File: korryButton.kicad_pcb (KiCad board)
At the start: 2 copper layers, 30 x 30 mm, 15 parts, among them CN1 B2B-XH-A (LF)(SN), CN2 B2B-XH-A (LF)(SN), SW1 5.8 ZSGT, U1 SN74AHCT125DR, U2 B3B-XH-A(LF)(SN), U3 WS2811C, U4 WS2811C

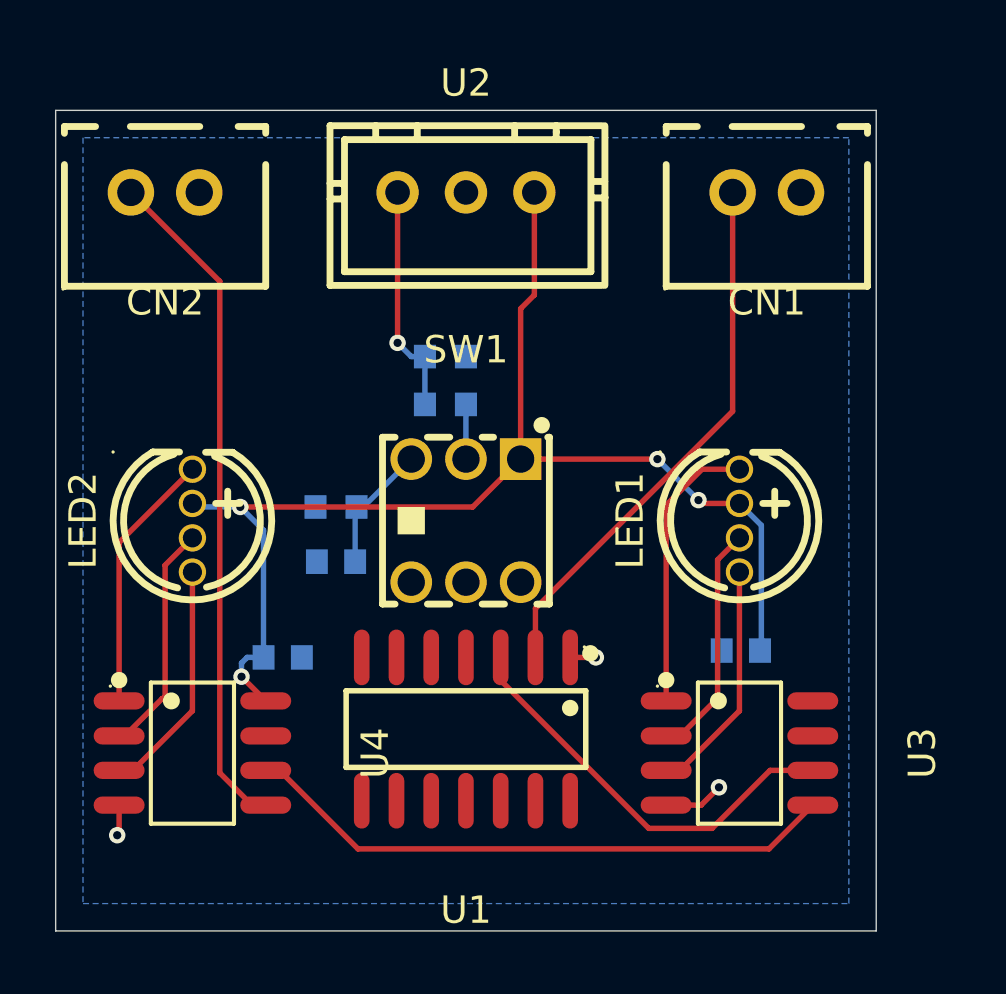
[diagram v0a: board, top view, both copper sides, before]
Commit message: update pcb
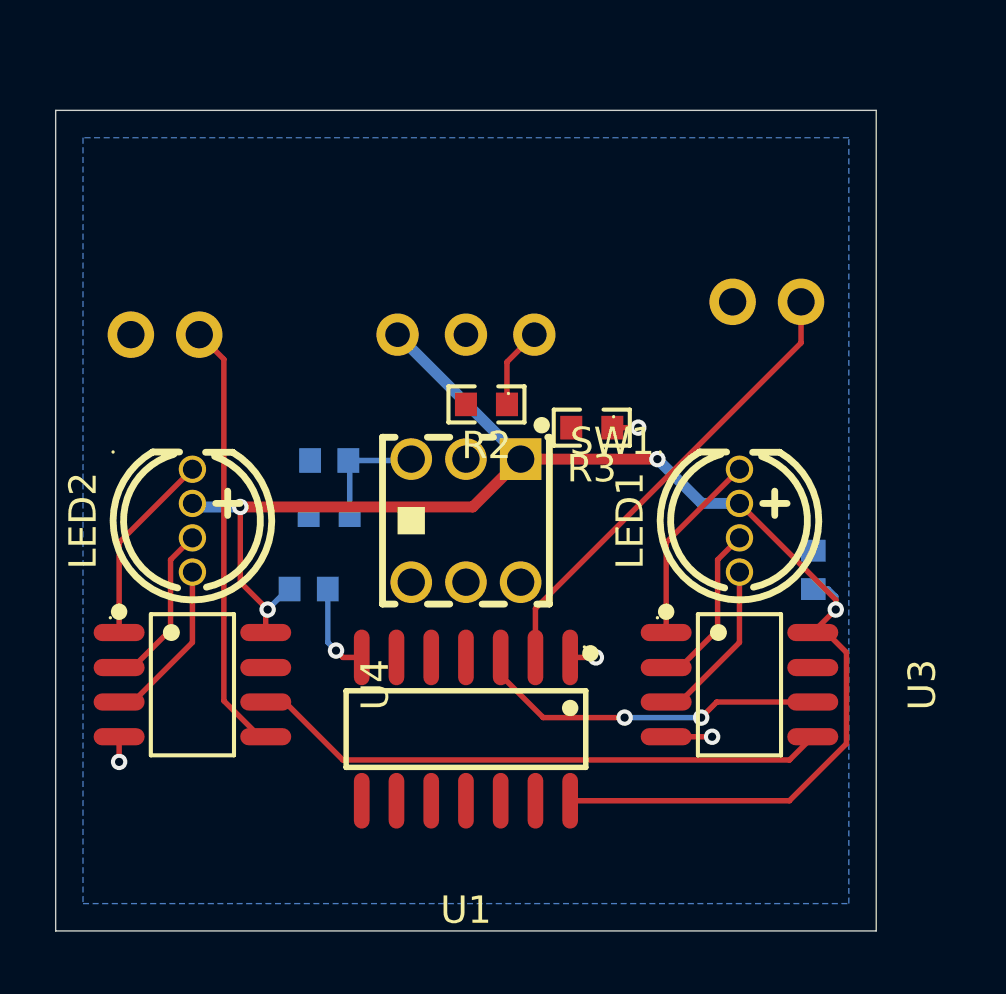
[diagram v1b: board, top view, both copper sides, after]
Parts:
- CN1, CN2, U2: moved to B.Cu
- R2, R3: moved to F.Cu
- moved R3 5.95 mm to (104.6, 121.6)
- moved CN2 5.20 mm to (89.0, 118.2), turned to 0 degrees
- moved U2 5.20 mm to (100.0, 118.2), turned to 180 degrees
- moved CN1 4.00 mm to (111.0, 117.0), turned to 0 degrees
- moved C3 3.97 mm to (112.7, 126.8), turned to -90 degrees
- moved C1 3.71 mm to (95.0, 122.8)
- moved C2 2.67 mm to (94.2, 127.5)
- moved U3 2.50 mm to (110.0, 131.0)
- moved U4 2.50 mm to (90.0, 131.0)
- moved R2 1.50 mm to (100.8, 120.8), turned to 180 degrees
- moved R1 0.39 mm to (95.0, 124.8)
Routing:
- net VCC: track 45.6 -> 58.0 mm
- net Net-(U4-DO): track 24.7 -> 15.8 mm
- net Net-(R2-Pad1): track 8.46 -> 2.96 mm, vias 1 -> 0
- net GND: track 4.49 -> 7.91 mm, vias 3 -> 5
- net Net-(LED1-R): track 10.4 -> 7.08 mm
- net Net-(U1-1A): track 20.0 -> 17.0 mm
- net Net-(LED1-G): track 8.64 -> 6.14 mm
- net Net-(LED2-R): track 9.58 -> 7.08 mm
- net Net-(LED2-B): track 8.65 -> 6.15 mm
- net Net-(LED1-B): track 8.65 -> 6.15 mm
- net Net-(U1-1Y): track 15.4 -> 12.9 mm, vias 0 -> 2
- net Net-(LED2-G): track 8.53 -> 6.14 mm
- net Net-(R2-Pad2): track 2.00 -> 0.00 mm
- net Net-(U3-DO): track 21.9 -> 21.2 mm
